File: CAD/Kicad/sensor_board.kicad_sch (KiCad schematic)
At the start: 7 parts, among them J2 RJ12_Shielded, U1 MPU-9250, U2 BME680

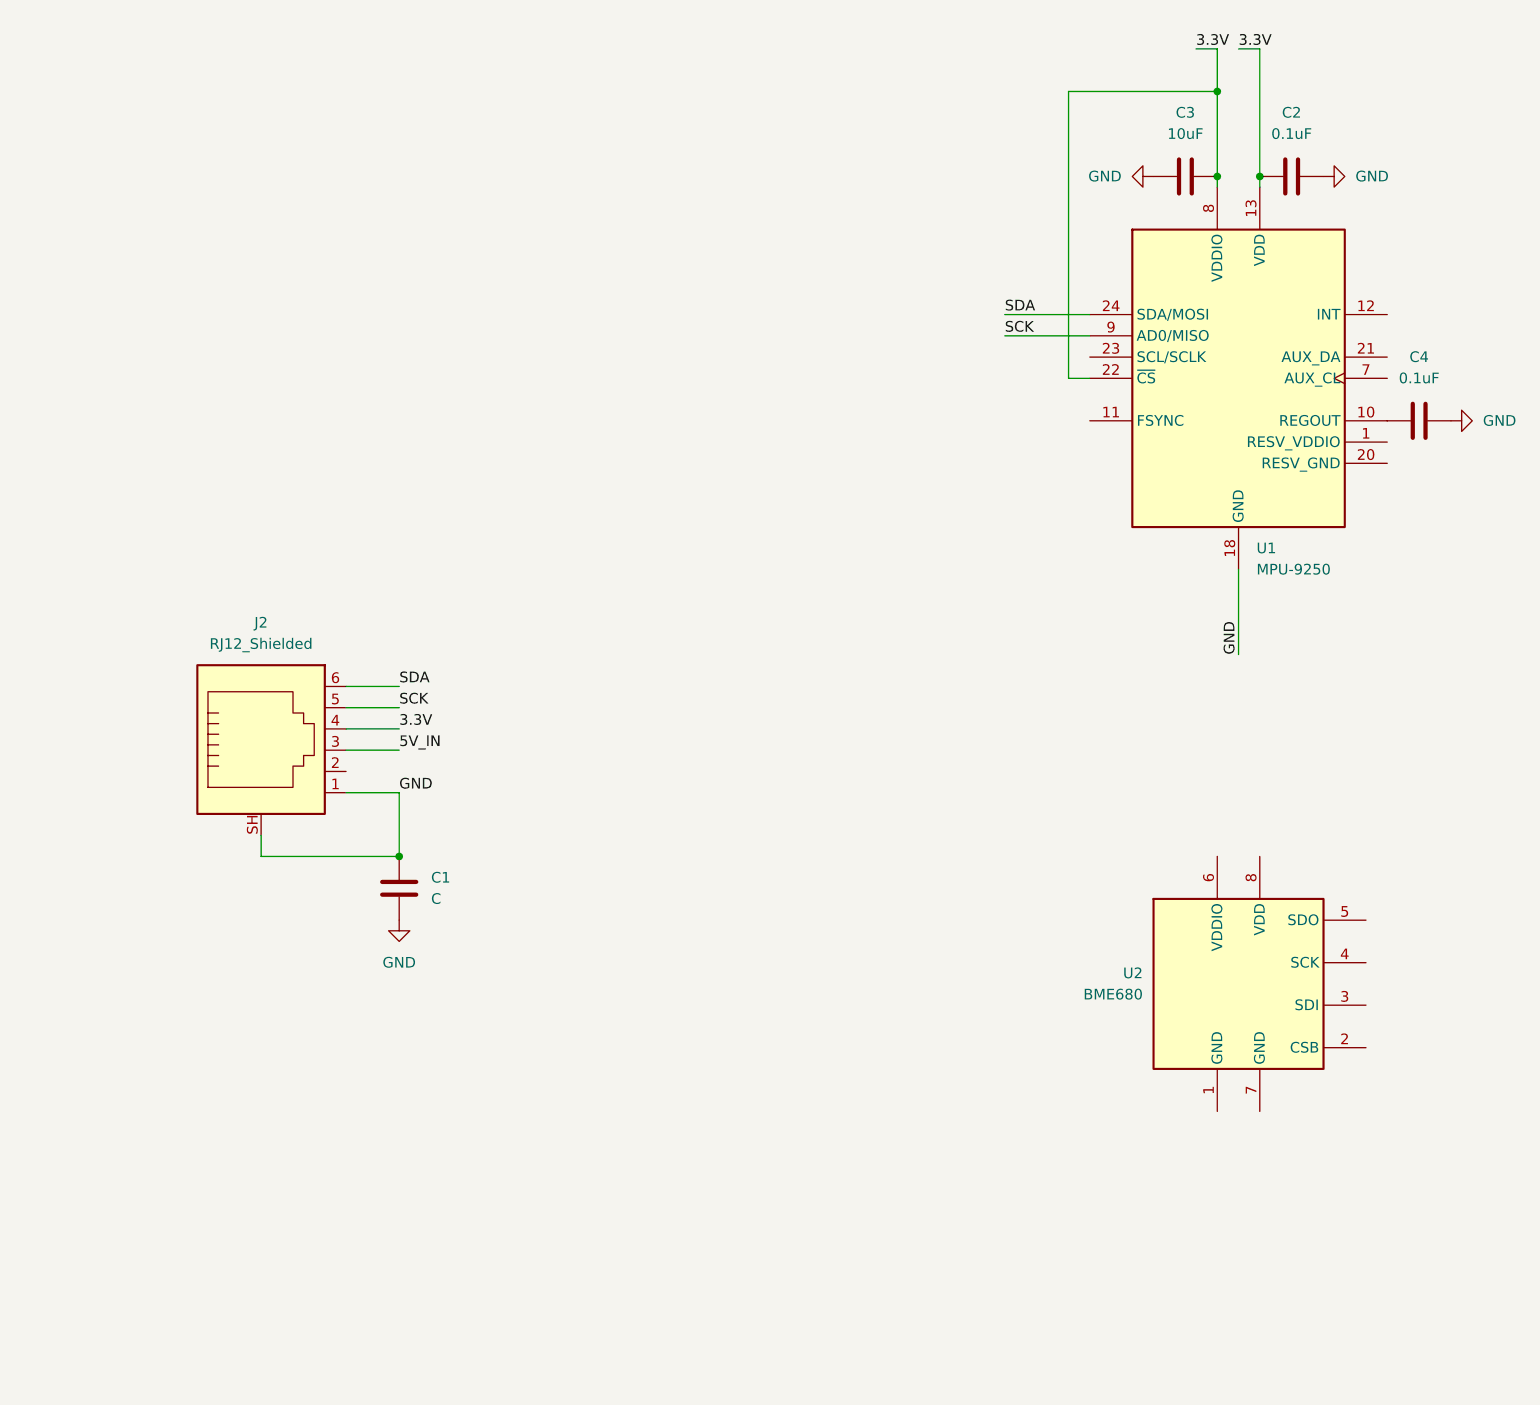
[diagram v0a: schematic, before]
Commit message: sensing revisions
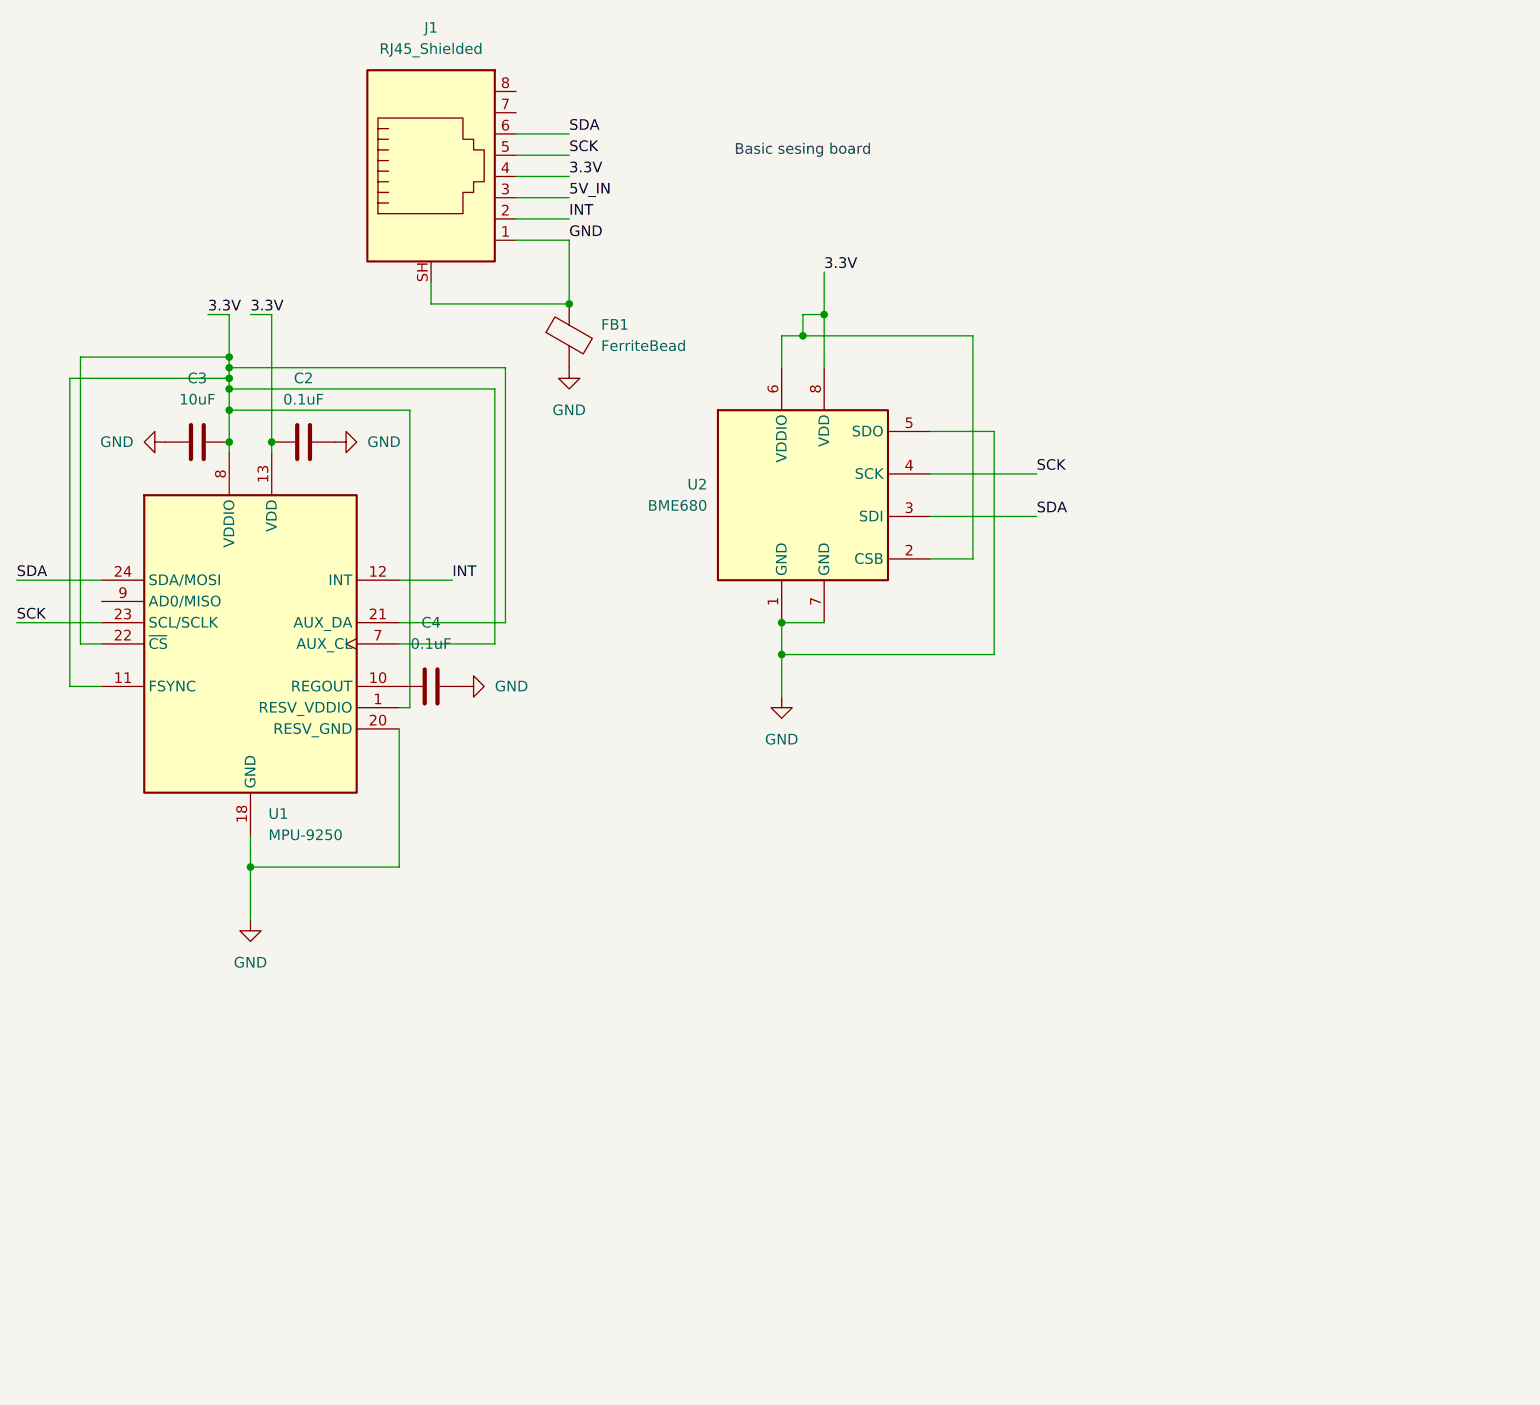
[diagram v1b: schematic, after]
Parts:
- removed C1: C, symbol Device:C
- removed J2: RJ12_Shielded, symbol Connector:RJ12_Shielded
- added FB1: FerriteBead, symbol Device:FerriteBead
- added J1: RJ45_Shielded, symbol Connector:RJ45_Shielded
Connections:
- net 3.3V: now also U1.1 (RESV_VDDIO), U1.11 (FSYNC), U1.21 (AUX_DA), U1.7 (AUX_CL), U2.2 (CSB), U2.6 (VDDIO), U2.8 (VDD), J1.4
- net 5V_IN: now also J1.3
- net GND: now also U1.20 (RESV_GND), U2.1 (GND), U2.5 (SDO), U2.7 (GND), FB1.1, FB1.2, J1.1, J1.SH
- net SCK: now also U1.23 (SCL/SCLK), U2.4 (SCK), J1.5; no longer U1.9 (AD0/MISO)
- net SDA: now also U2.3 (SDI), J1.6
- net INT: now reaches U1.12 (INT)
- net INT: now also J1.2
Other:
- note added: "Basic sesing board"
- moved on the sheet: C2, C3, C4, U1, U2

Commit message: Journal entry and small PCB tweaks
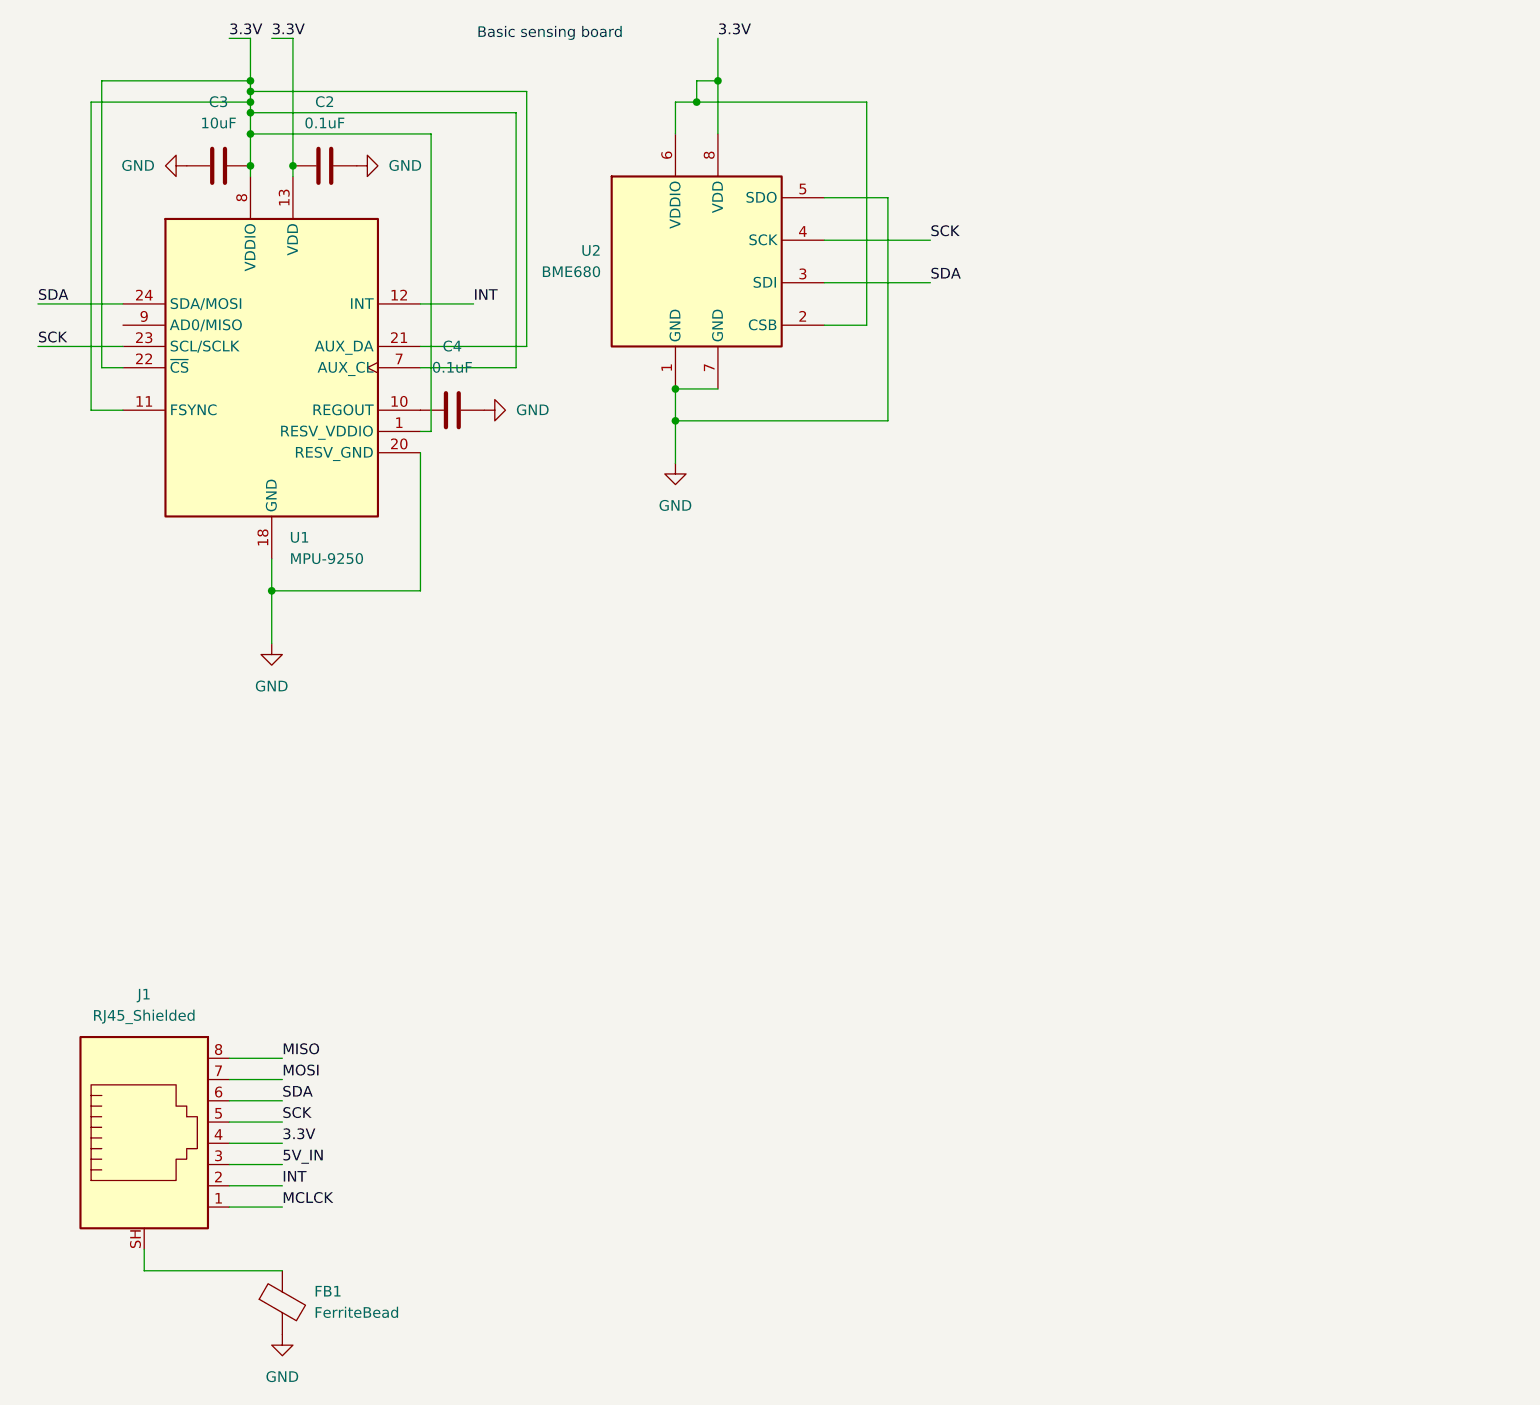
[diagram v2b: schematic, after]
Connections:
- net GND: no longer FB1.1, J1.1, J1.SH
- net MOSI: now reaches J1.7
- net MISO: now reaches J1.8
- new net: FB1.1, J1.SH
- new net MCLCK: J1.1
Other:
- note added: "Basic sensing board"
- note removed: "Basic sesing board"
- moved on the sheet: C2, C3, C4, FB1, J1, U1, U2
